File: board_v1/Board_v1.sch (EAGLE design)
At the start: 38 parts, among them IC1 MAX7219, IC2 MAX7219, IC3 MAX7219, SW1 ROTARY SWITCH

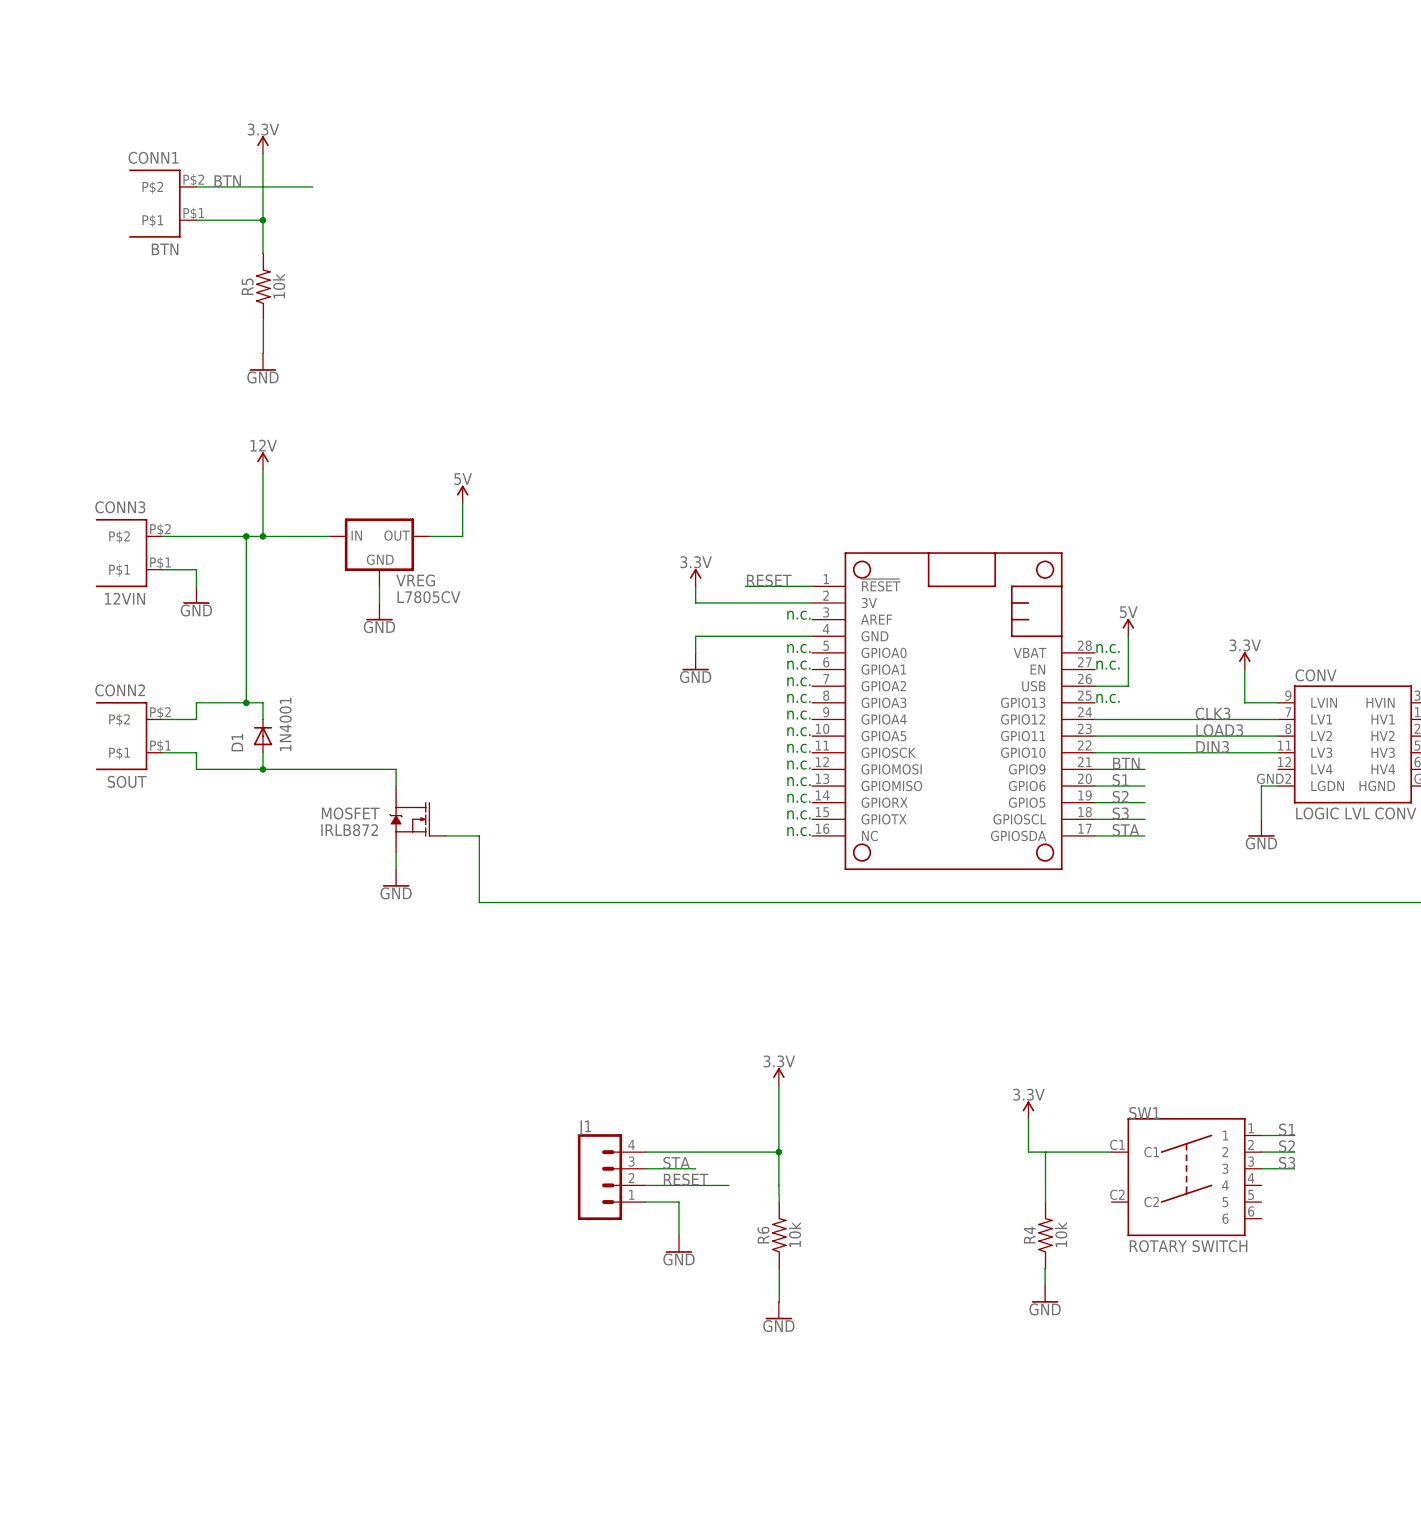
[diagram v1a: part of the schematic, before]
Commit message: more pull down updates
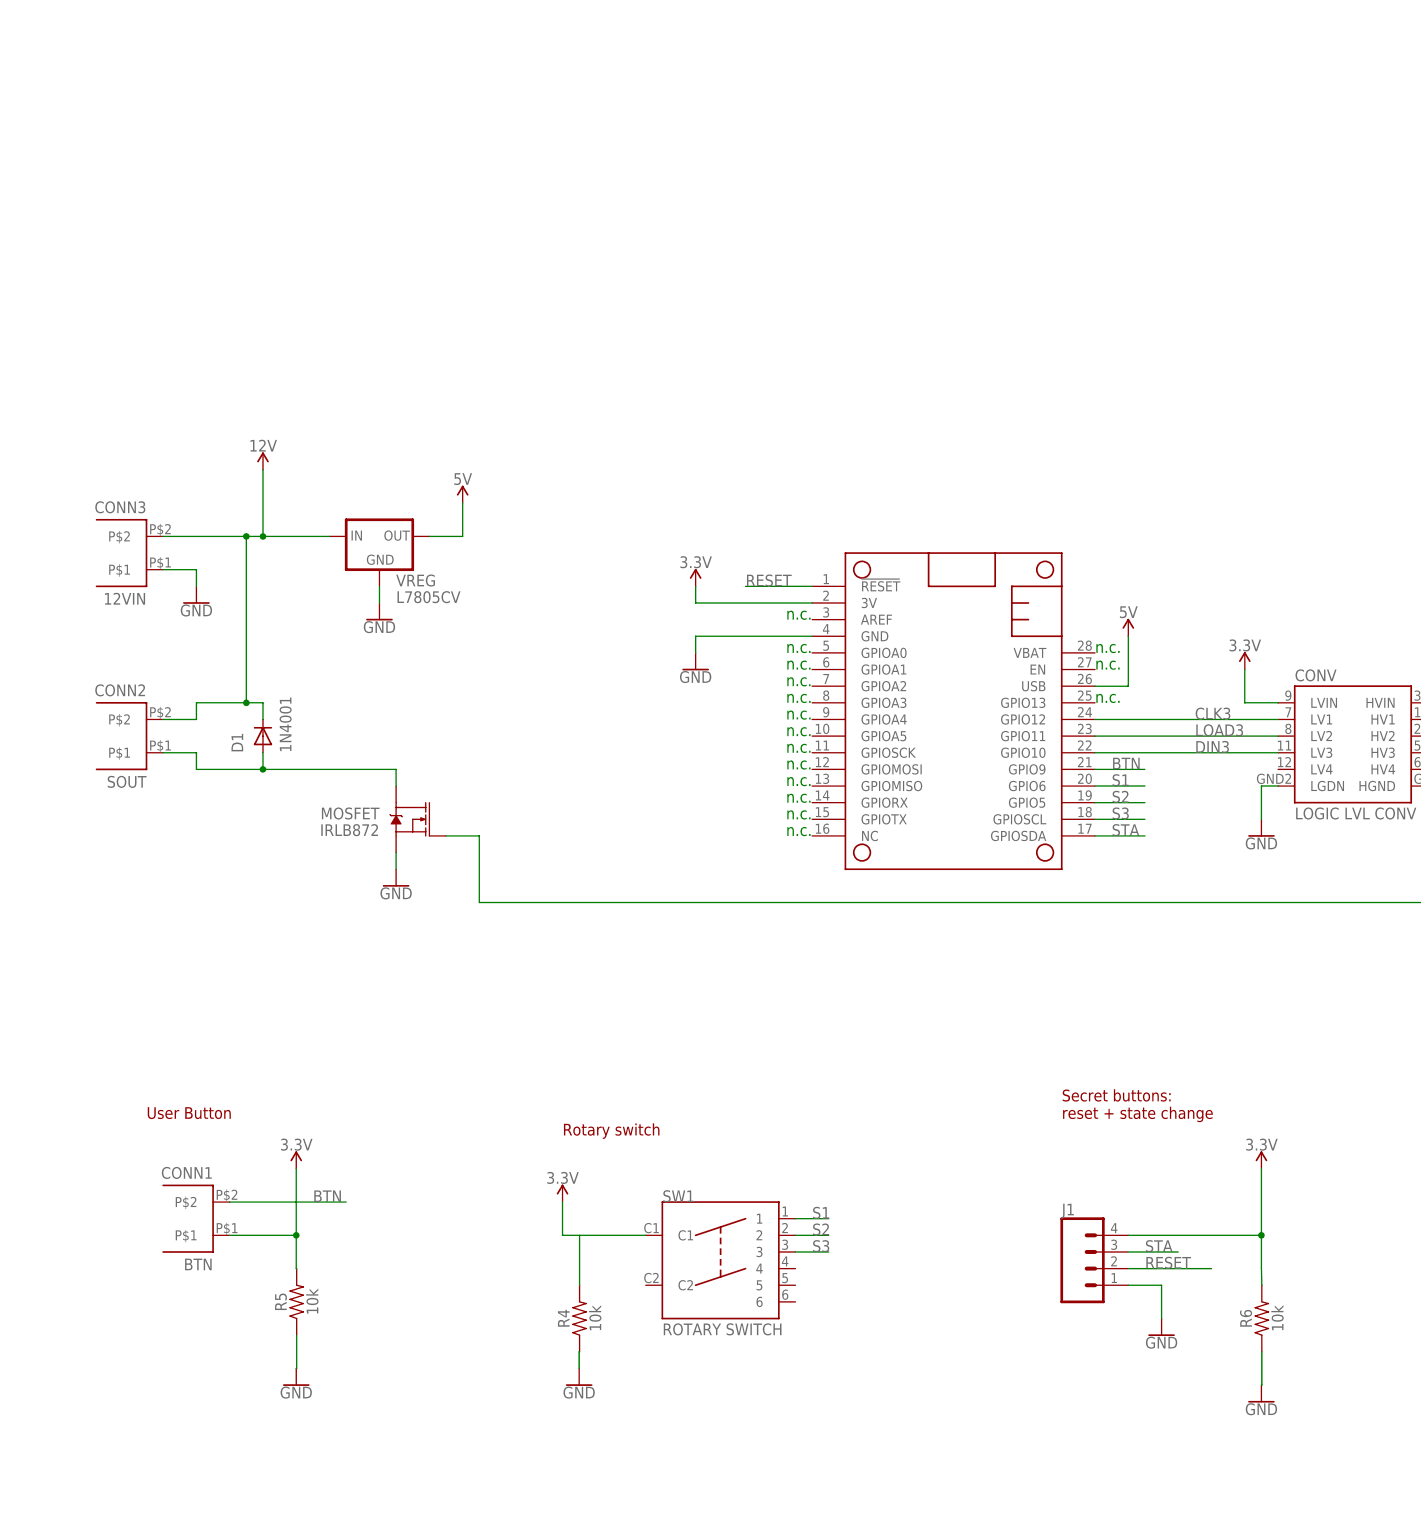
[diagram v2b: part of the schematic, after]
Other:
- note added: "Rotary switch"
- note added: "Secret buttons: reset + state change"
- note added: "User Button"
- moved on the sheet: BTN, J1, R4, R5, R6, SW1
